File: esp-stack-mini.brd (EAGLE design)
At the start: 81.8 x 81.8 mm, 62 parts, among them IC1 FT232RL, Q1 BSS138, Q2 AO3401, Q3 S8050, Q4 S8050, U1 TPS737XX, U2 MCP73831

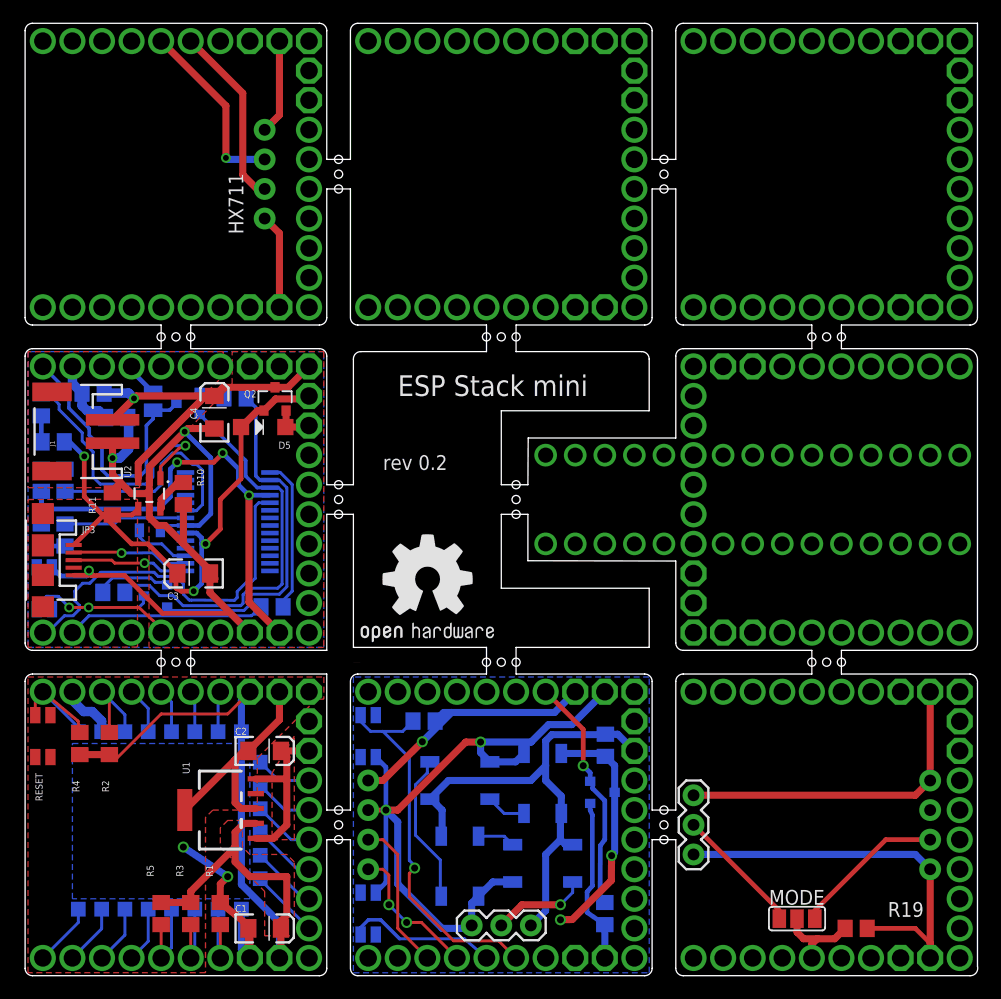
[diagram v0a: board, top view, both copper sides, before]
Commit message: wip
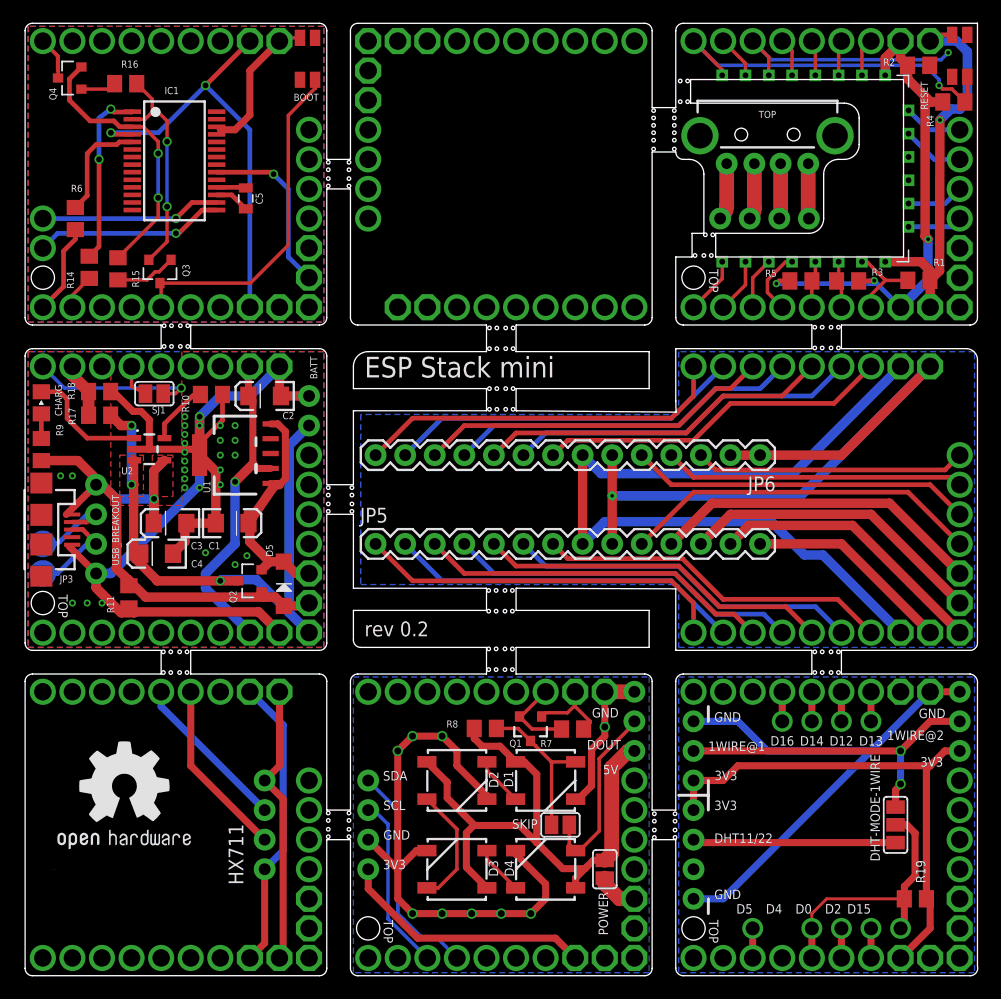
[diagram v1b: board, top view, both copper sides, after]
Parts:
- removed 1WIRE: (no value), SparkFun-Connectors:1X03
- removed B1, B2: (no value), ESPStack-mini:SKSCLDE010
- removed CHARGING: DIODE_SMDD0805, diodes_gen:D0805
- removed D7: TX, diodes_gen:D0805
- removed D8: RX, diodes_gen:D0805
- removed J1: (no value), SparkFun-Connectors:JST-2-SMD
- removed MODE: (no value), SparkFun-Retired:SJ_2
- removed R12, R13: 10k, resistor:R0805
- added 1WIRE@1, 1WIRE@2: (no value), SparkFun-Connectors:1X03_NO_SILK
- added BATT: (no value), SparkFun-Connectors:1X02_NO_SILK
- added CHARG: DIODE_SMDD0805, diodes_gen:D0805
- added DHT-MODE-1WIRE: (no value), SparkFun-Retired:SJ_2
- added JP4: USB-A-H, SparkFun-Connectors:USB-A-H
- added JP5, JP6: (no value), SparkFun-Connectors:1X14
- added POWER, SKIP: (no value), jumper:SJ
- added U$2, U$3: POGO-PAD, ESPStack-mini:POGO-PAD
- added USB_BREAKOUT, USB_BREAKOUT1: (no value), SparkFun-Connectors:1X04_NO_SILK_ALL_ROUND
- JP2: device SparkFun-Connectors:1X03 -> SparkFun-Connectors:1X03_NO_SILK
- R19: value 9k1 -> 4k7*
- R6: value 10k -> 470
- moved RESET 98.0 mm to (80.0, 78.7), turned to 90 degrees
- moved R4 93.1 mm to (79.5, 74.8), turned to 180 degrees
- moved R2 90.7 mm to (76.5, 77.9), turned to 180 degrees
- moved R1 81.0 mm to (76.5, 59.5), turned to 180 degrees
- moved H1 79.0 mm to (55.9, 55.9)
- moved ESP-12E 78.7 mm to (75.6, 61.1)
- moved R3 78.3 mm to (70.4, 59.4), turned to 0 degrees
- moved R5 77.3 mm to (66.4, 59.4), turned to 180 degrees
- moved H4 55.9 mm to (0.00, 0.00)
- moved HX711 55.9 mm to (20.3, 8.89)
- moved R6 52.5 mm to (4.06, 64.8), flipped to the top, turned to 90 degrees
- moved BOOT 50.8 mm to (24.0, 78.5), flipped to the top
- moved H6 35.9 mm to (55.9, 27.9), turned to 0 degrees
- moved C1 34.9 mm to (17.5, 38.6)
- moved R14 33.1 mm to (5.26, 60.6), flipped to the top, turned to 90 degrees
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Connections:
- removed net S1: H1.S1, H6.S1, H7.S1, H8.S1
- new net N$40: H6.D0, JP5.5
- new net N$52: H6.D2, JP5.6
- new net N$58: H6.D15, JP5.7
- new net N$65: H6.RST, JP6.14
- new net N$66: H6.ADC, JP6.13
- new net N$67: H6.EN, JP6.12
- new net N$68: H6.D16, JP6.11
- new net N$69: H6.D14, JP6.10
- new net N$70: H6.D12, JP6.9
- new net N$71: H6.D13, JP6.8
- new net NEOPIXEL_EXTERNAL: D4.2, JP2.2, SKIP.2
- new net NEOPIXEL_VCC: D1.1, D2.1, D3.1, D4.1, JP2.3, POWER.1, R8.2
- new net VBAT: H6.VBATT, JP5.13
- net 1WIRE: now also 1WIRE@1.2, 1WIRE@2.2, DHT-MODE-1WIRE.3; no longer 1WIRE.2, MODE.3
- net 3V3: now also 1WIRE@1.1, 1WIRE@2.1, C2.A, JP5.8, JP6.7; no longer 1WIRE.1, C1.A, D7.A, D8.A, R6.2
- net ADC: no longer H6.ADC, H8.ADC
- net CS0: now also H6.CS0, JP6.3
- net D+: now also JP4.D+, U$3.P$2, USB_BREAKOUT.2, USB_BREAKOUT1.2
- net D-: now also JP4.D-, U$2.P$2, USB_BREAKOUT.3, USB_BREAKOUT1.3
- net D0: now also DHT-MODE-1WIRE.2; no longer B2.1, H6.D0, MODE.2
- net D10: no longer H1.D10, H6.D10, H7.D10, H8.D10
- net D12: now also H5.D12; no longer H6.D12, H8.D12
- net D13: now also H5.D13; no longer H6.D13, H8.D13
- net D14: now also H5.D14; no longer H6.D14, H8.D14
- net D15: now also H5.D15; no longer H6.D15, H8.D15
- net D16: now also H5.D16; no longer H6.D16, H8.D16
- net D2: now also H5.D2; no longer B1.2, H6.D2, H8.D2, R6.1
- net D4: now also H5.D4; no longer H6.D4, H8.D4
- net D5: now also H5.D5; no longer H6.D5, H8.D5
- net D9: no longer H1.D9, H6.D9, H7.D9, H8.D9
- net DHT: now also DHT-MODE-1WIRE.1; no longer MODE.1
- net GND: now also 1WIRE@1.3, 1WIRE@2.3, BATT.2, JP4.GND, JP5.14, JP5.9, JP6.1, JP6.2, JP6.6, USB_BREAKOUT.1, USB_BREAKOUT1.1; no longer 1WIRE.3, B1.3, B2.4, J1.1
- net MISO: now also H6.MISO, JP6.4
- net MOSI: now also H6.MOSI, JP6.5
- net N$17: now also H6.TX, JP5.1; no longer IC1.23, R12.2
- net N$18: now also H6.RX, JP5.2; no longer IC1.22, R13.2
- net N$19: now also H6.D5, JP5.3; no longer D7.K, R12.1
- net N$20: now also H6.D4, JP5.4; no longer D8.K, R13.1
- net N$4: now also IC1.5, R6.2; no longer D4.2, JP2.2
- net N$6: now also CHARG.A; no longer CHARGING.A
- net N$7: now also CHARG.K; no longer CHARGING.K
- net NEOPIXEL: now also SKIP.1
- net RST: now also H8.RST
- net RX: now also H8.RX
- net SCLK: now also H6.SCLK, JP5.10
- net TX: now also H8.TX, R6.1; no longer IC1.5
- net V+: now also C1.A, JP5.11, POWER.2; no longer C2.A, D1.1, D2.1, D3.1, D4.1, JP2.3, R8.2
- net VBATT: now also BATT.1; no longer H6.VBATT, J1.2
- net VBUS: now also JP4.VBUS, JP5.12, USB_BREAKOUT.4, USB_BREAKOUT1.4
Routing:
- net GND: track 213.3 -> 361.3 mm, vias 7 -> 39
- net 3V3: track 189.5 -> 281.6 mm, vias 4 -> 6
- net NEOPIXEL_VCC: track 0.00 -> 52.7 mm
- net VBUS: track 51.2 -> 98.6 mm, vias 3 -> 2
- net D2: track 39.8 -> 6.80 mm
- net N$65: track 0.00 -> 31.9 mm
- net N$67: track 0.00 -> 30.5 mm
- net N$71: track 0.00 -> 30.5 mm
- net N$69: track 0.00 -> 30.5 mm
- net N$66: track 0.00 -> 30.5 mm
- net N$58: track 0.00 -> 30.5 mm
- net N$40: track 0.00 -> 30.5 mm, vias 1 -> 0
- net N$70: track 0.00 -> 30.5 mm
- net N$68: track 0.00 -> 30.5 mm
- net N$52: track 0.00 -> 30.5 mm, vias 1 -> 0
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- removed copper zone on layer 1, net 3V3
- removed copper zone on layer 1, net V+
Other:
- outline, holes or cut-outs redrawn
- board text added: "5V"
- board text added: "D0"
- board text added: "D12"
- board text added: "D13"
- board text added: "D14"
- board text added: "D15"
- board text added: "D16"
- board text added: "D2"
- board text added: "D4"
- board text added: "D5"
- board text added: "DOUT"
- board text added: "TOP"
- board text removed: "DIN"
- board text removed: "VBUS"
- board text removed: "breadboard adapter"
- board text removed: "esp-12e"
